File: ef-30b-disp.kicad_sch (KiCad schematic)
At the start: 20 parts, among them J1 Conn_01x04, J1 IC16, J2 IC16

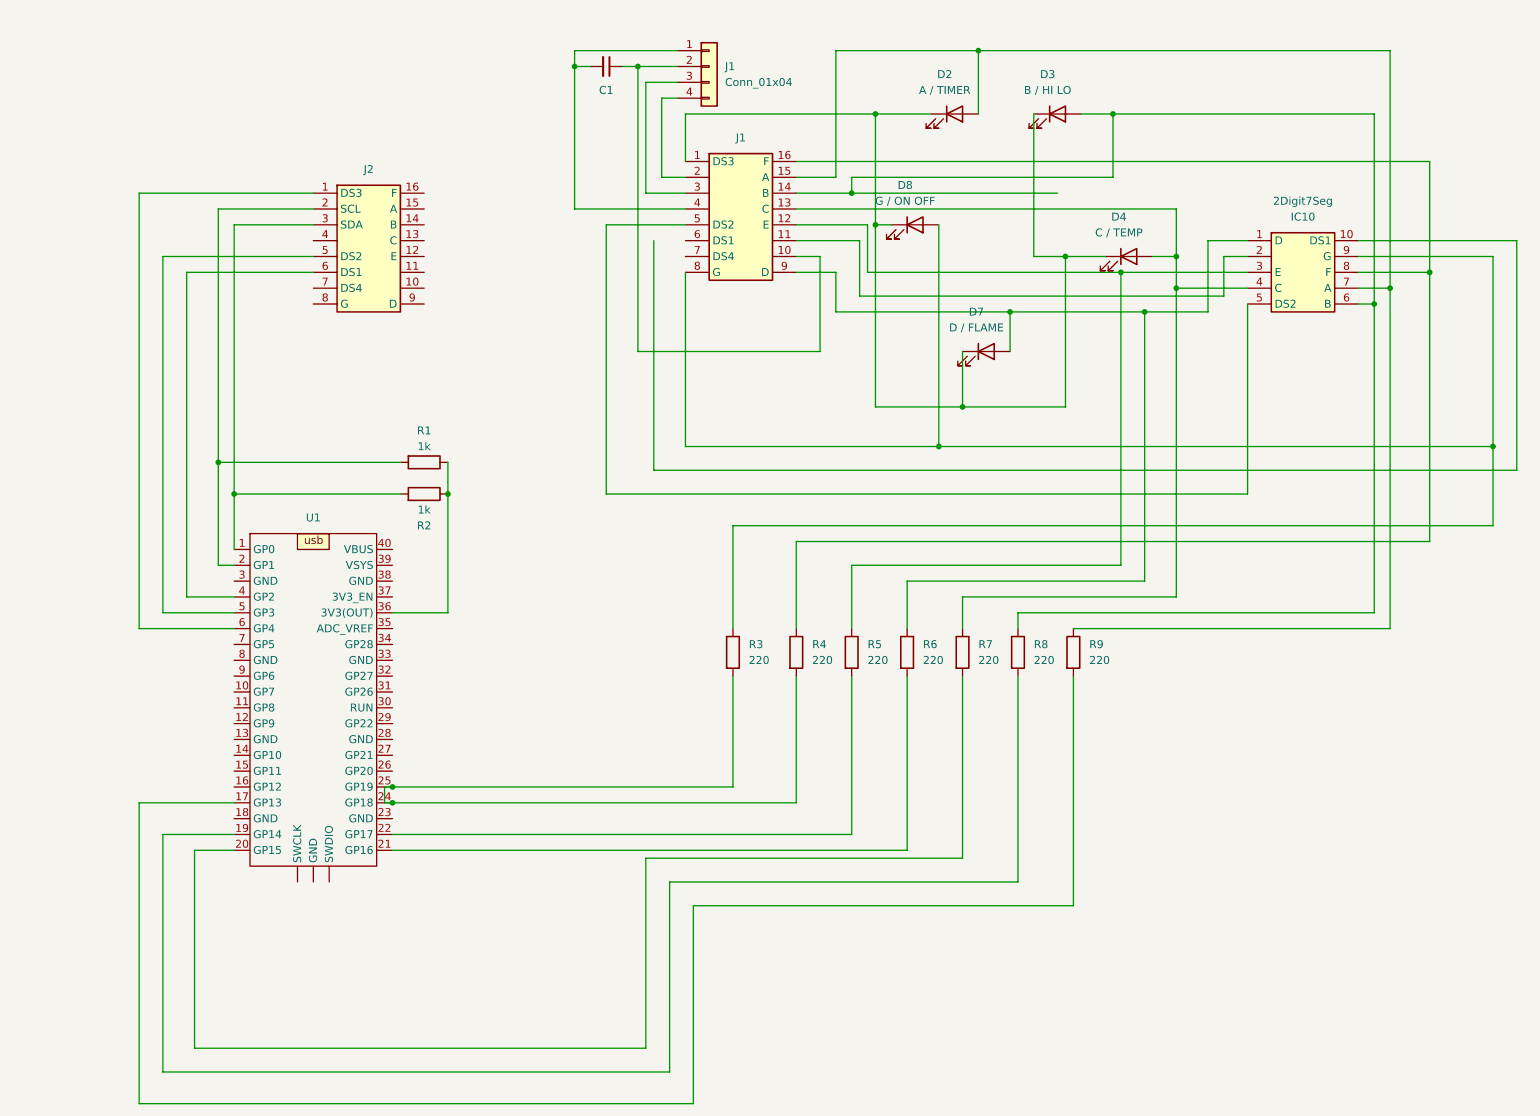
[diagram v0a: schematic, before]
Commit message: Updated the schematic.
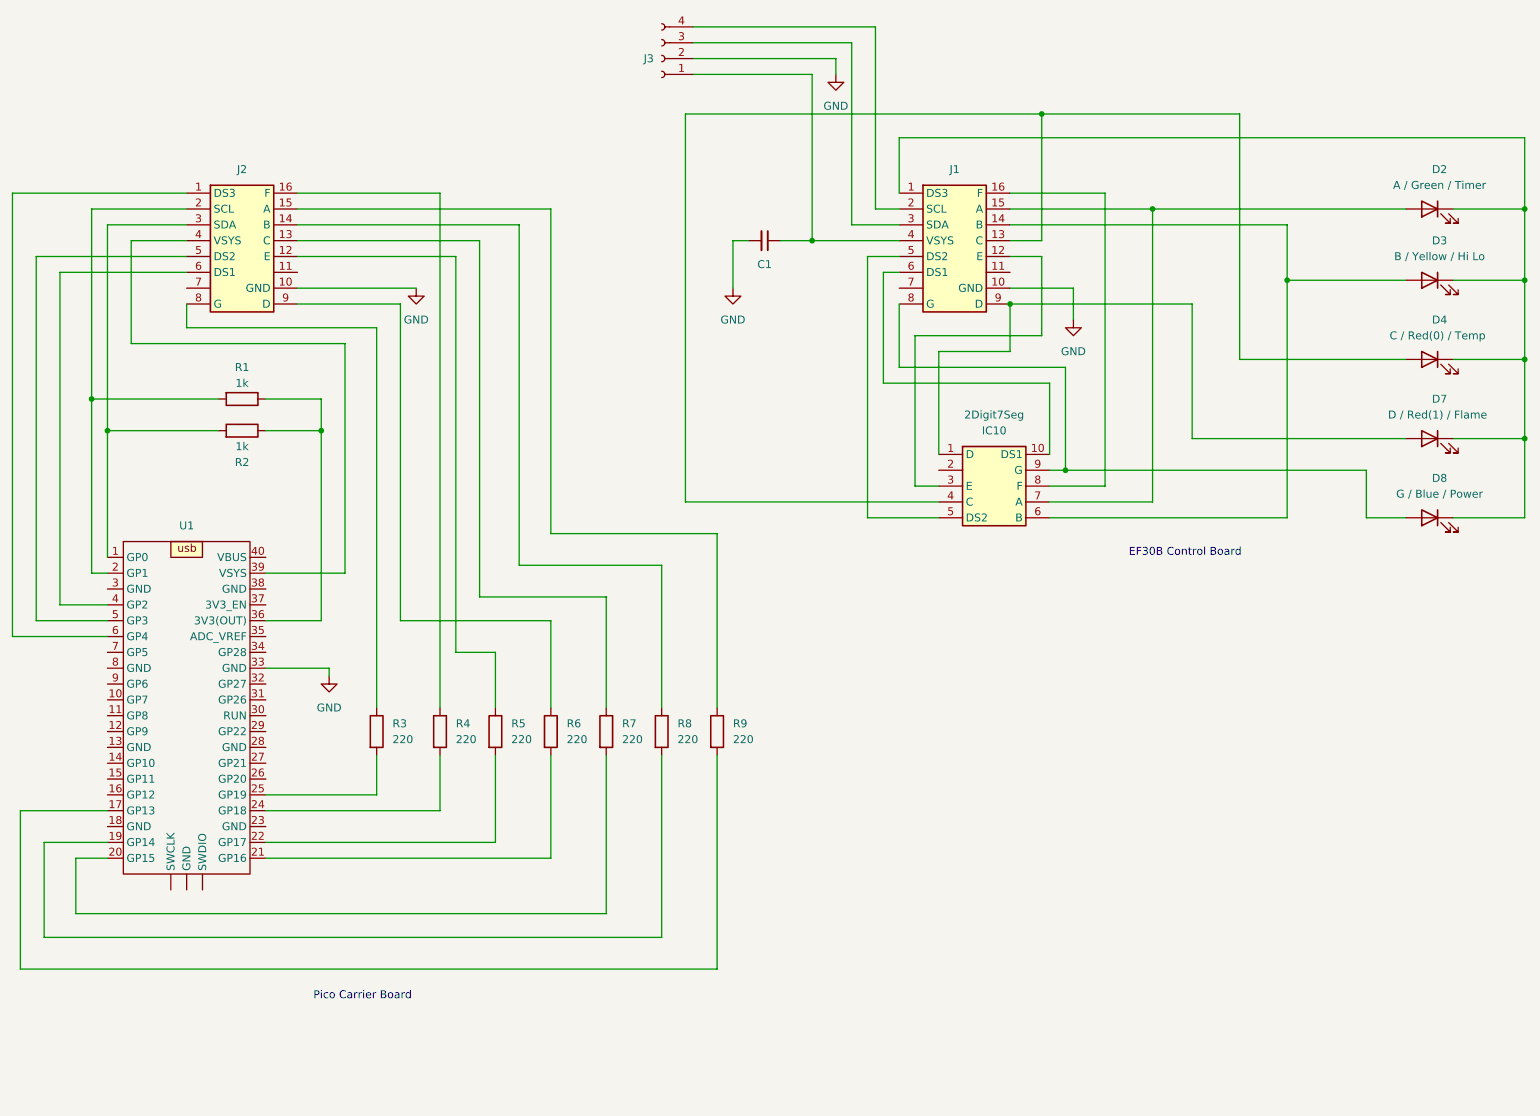
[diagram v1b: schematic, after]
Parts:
- removed J1: IC16, symbol Generic IC:IC16
- added J3: ~, symbol Connector:Conn_01x04_Socket
- D2: value A / TIMER -> A / Green / Timer
- D3: value B / HI LO -> B / Yellow / Hi Lo
- D4: value C / TEMP -> C / Red(0) / Temp
- D7: value D / FLAME -> D / Red(1) / Flame
- D8: value G / ON OFF -> G / Blue / Power
- J1: value Conn_01x04 -> IC16
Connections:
- net at D2.1 (K), D3.1 (K), D4.1 (K)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: now also J1.1 (DS3)
- net at 2Digit7Seg.6 (B), D3.2 (A): now also J1.14 (B); no longer R8.1
- net at 2Digit7Seg.7 (A), D2.2 (A): now also J1.15 (A); no longer R9.1
- net at 2Digit7Seg.1 (D), D7.2 (A): now also J1.9 (D); no longer R6.1
- net at R4.1: now also J2.16 (F); no longer 2Digit7Seg.8 (F)
- net at R4.2, U1.24 (GP18): no longer R3.2, U1.25 (GP19)
- net at C1.1: now also J1.4 (VSYS), J3.1 (Pin_1); no longer J1.2 (Pin_2)
- net GND: now reaches C1.2
- net GND: now also J1.10 (GND), J2.10 (GND), U1.33 (GND), J3.2 (Pin_2); no longer J1.1 (Pin_1)
- net at 2Digit7Seg.10 (DS1): now also J1.6 (DS1)
- net at 2Digit7Seg.3 (E): now also J1.12 (E); no longer R5.1
- net at 2Digit7Seg.4 (C), D4.2 (A): now also J1.13 (C); no longer R7.1
- net at 2Digit7Seg.5 (DS2): now also J1.5 (DS2)
- net at 2Digit7Seg.9 (G), D8.2 (A): now also J1.8 (G); no longer R3.1
- net at U1.39 (VSYS): now also J2.4 (VSYS)
- net at J1.3 (SDA): now also J3.3 (Pin_3)
- net at J2.12 (E): now also R5.1
- net at J2.13 (C): now also R7.1
- net at J2.14 (B): now also R8.1
- net at J2.15 (A): now also R9.1
- net at J2.8 (G): now also R3.1
- net at J2.9 (D): now also R6.1
- new net: 2Digit7Seg.8 (F), J1.16 (F)
- new net: R3.2, U1.25 (GP19)
- new net: J1.2 (SCL), J3.4 (Pin_4)
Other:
- note added: "EF30B Control Board"
- note added: "Pico Carrier Board"
- moved on the sheet: 2Digit7Seg, C1, D2, D3, D4, D7, D8, R1, R2, R3, R4, R5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
